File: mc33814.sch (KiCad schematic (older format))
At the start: 1 part, among them U11 MC33814

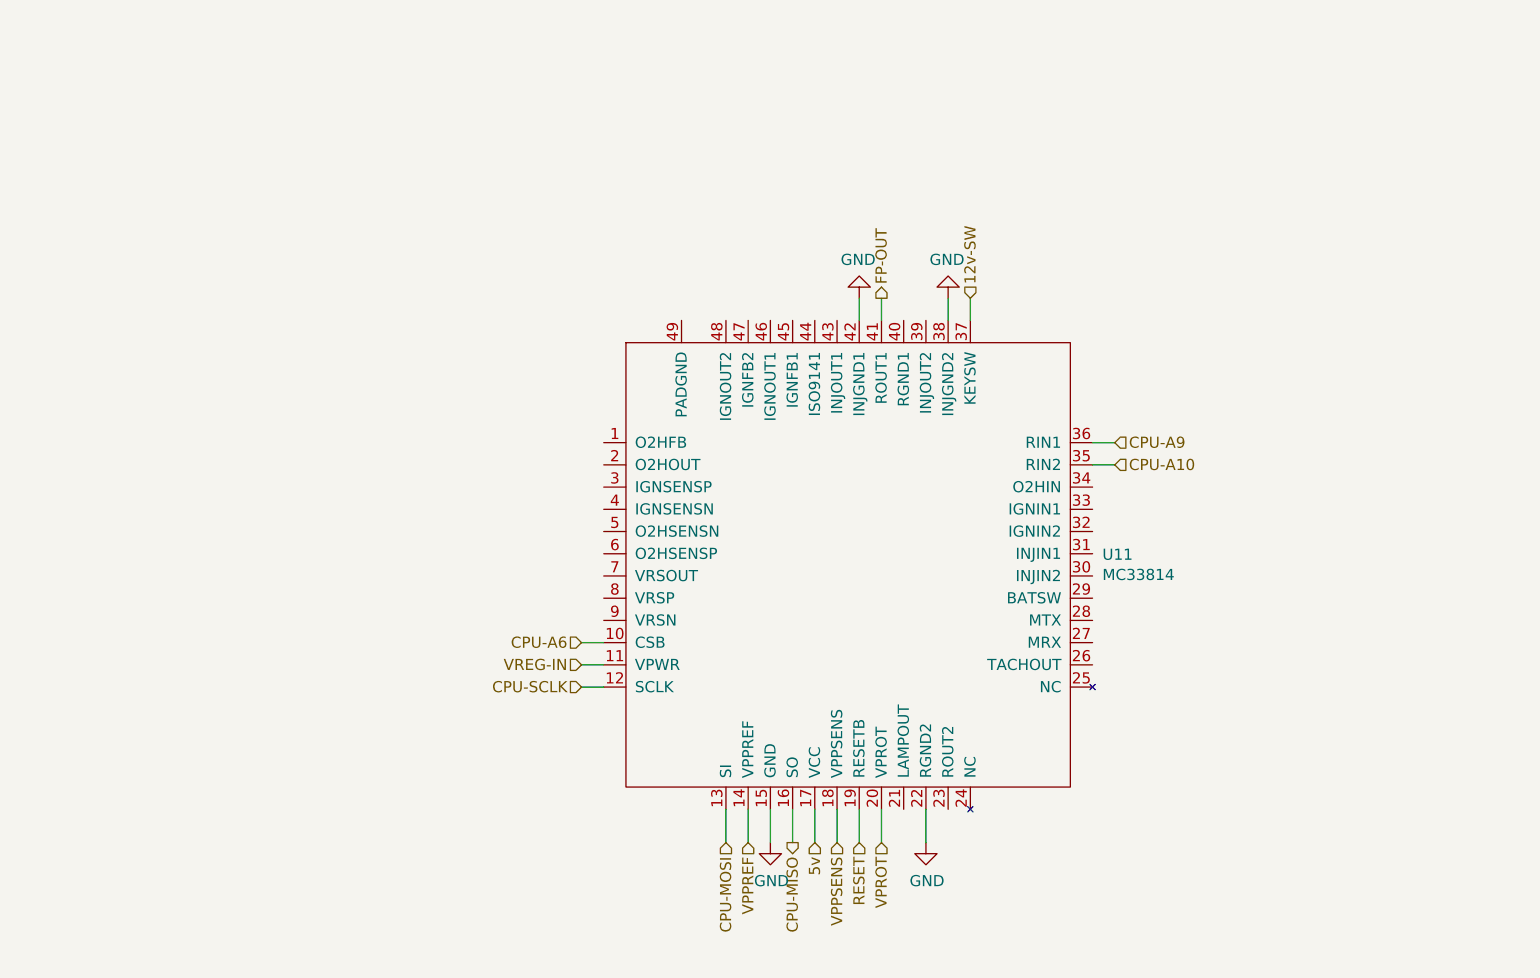
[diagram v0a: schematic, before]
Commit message: restart a third time
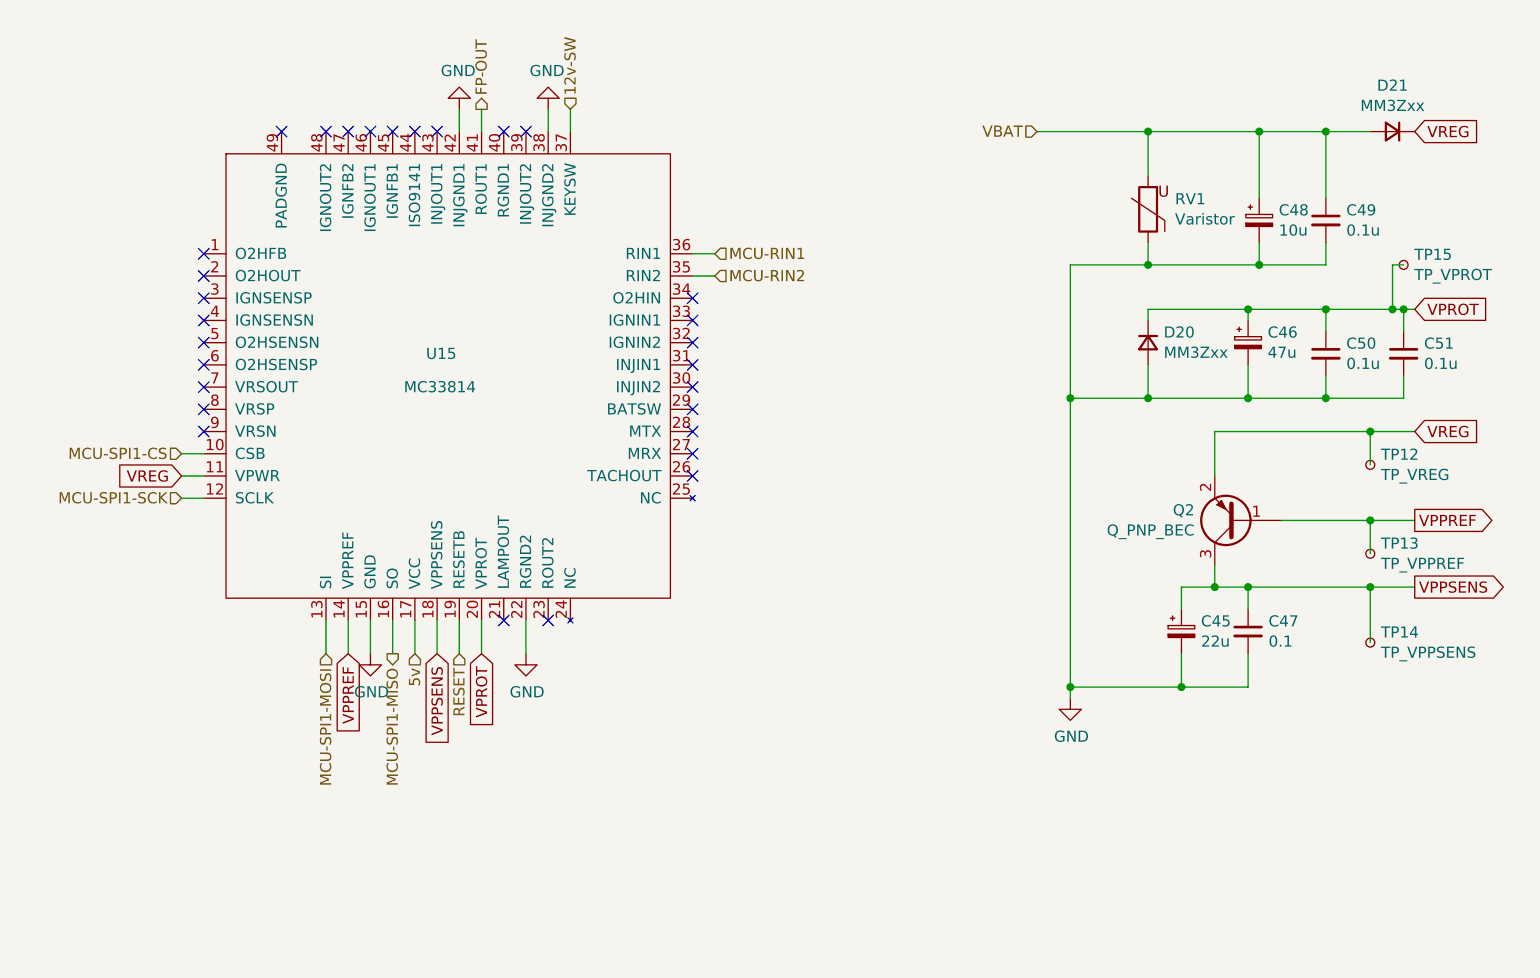
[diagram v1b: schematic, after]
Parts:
- added C45: 22u, Capacitor_SMD:CP_Elec_4x4.5, symbol Device:CP_Small
- added C46: 47u, Capacitor_SMD:CP_Elec_5x5.8, symbol Device:CP_Small
- added C47: 0.1, Capacitor_SMD:C_0805_2012Metric_Pad1.18x1.45mm_HandSolder, symbol Device:C_Small
- added C48: 10u, Capacitor_Tantalum_SMD:CP_EIA-7343-20_Kemet-V_Pad2.25x2.55mm_HandSolder, symbol Device:CP_Small
- added C49, C50, C51: 0.1u, Capacitor_SMD:C_1206_3216Metric_Pad1.33x1.80mm_HandSolder, symbol Device:C_Small
- added D20, D21: MM3Zxx, Diode_SMD:D_SOD-323_HandSoldering, symbol Device:D_Small
- added Q2: Q_PNP_BEC, Package_TO_SOT_SMD:SOT-23, symbol Device:Q_PNP_BEC
- added RV1: Varistor, Varistor:RV_Disc_D15.5mm_W3.9mm_P7.5mm, symbol Device:Varistor
- added TP12: TP_VREG, TestPoint:TestPoint_Pad_D1.0mm, symbol Connector:TestPoint_Small
- added TP13: TP_VPPREF, TestPoint:TestPoint_Pad_D1.0mm, symbol Connector:TestPoint_Small
- added TP14: TP_VPPSENS, TestPoint:TestPoint_Pad_D1.0mm, symbol Connector:TestPoint_Small
- added TP15: TP_VPROT, TestPoint:TestPoint_Pad_D1.0mm, symbol Connector:TestPoint_Small
- renumbered U11 to U15
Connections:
- net GND: now also C45.2, C46.2, C47.2, C48.2, C49.2, C50.2, C51.2, D20.2 (A), RV1.1
- net VPPREF: now also Q2.1 (B), TP13.1
- net VPPSENS: now also C45.1, C47.1, Q2.3 (C), TP14.1
- net VPROT: now also C46.1, C50.1, C51.1, D20.1 (K), TP15.1
- net CPU-A10 renamed MCU-RIN2
- net CPU-A6 renamed MCU-SPI1-CS
- net CPU-A9 renamed MCU-RIN1
- net CPU-MISO renamed MCU-SPI1-MISO
- net CPU-MOSI renamed MCU-SPI1-MOSI
- net CPU-SCLK renamed MCU-SPI1-SCK
- net VREG-IN renamed VREG
- net VREG: now also D21.1 (K), Q2.2 (E), TP12.1
- new net VBAT: C48.1, C49.1, D21.2 (A), RV1.2
- no-connect marks 0 -> 29
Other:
- moved on the sheet: U15
